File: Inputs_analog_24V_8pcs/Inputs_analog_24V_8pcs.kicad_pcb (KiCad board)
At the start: 2 copper layers, 104 parts, among them J1 Screw_Terminal_01x02, J10 Screw_Terminal_01x03, J11 Screw_Terminal_01x03, J2 Screw_Terminal_01x02, J3 Screw_Terminal_01x06, J4 Screw_Terminal_01x03, J5 Screw_Terminal_01x03, J6 Screw_Terminal_01x03, J7 Screw_Terminal_01x03, J8 Screw_Terminal_01x03, J9 Screw_Terminal_01x03, U1 SN74HC14N, U10 4N28, U11 4N28, U2 SN74HC14N, U3 74HC151N.652, U4 4N28, U5 4N28, U6 4N28, U7 4N28, U8 4N28, U9 4N28

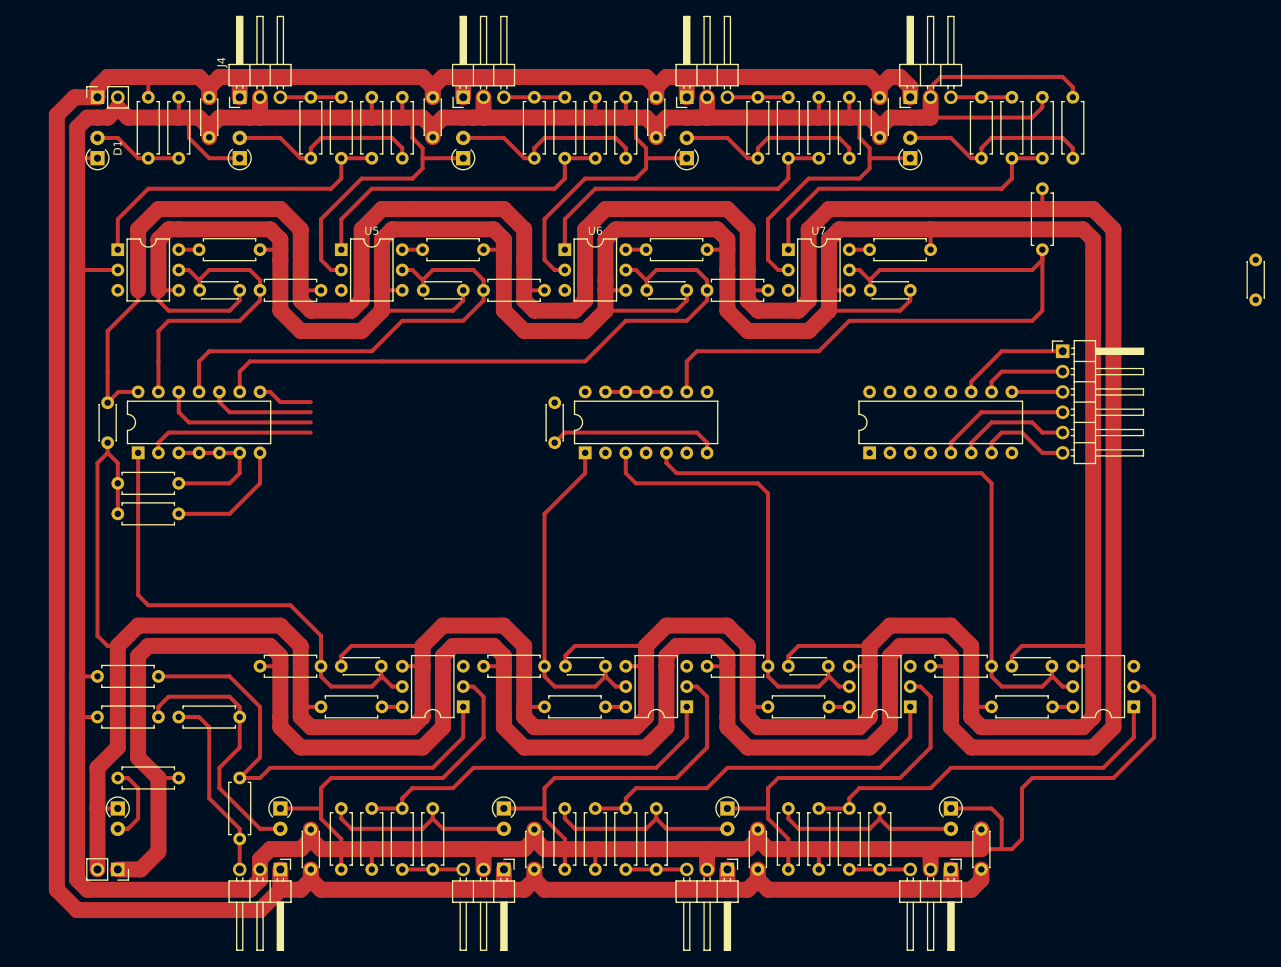
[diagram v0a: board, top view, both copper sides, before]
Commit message: Finish pcb
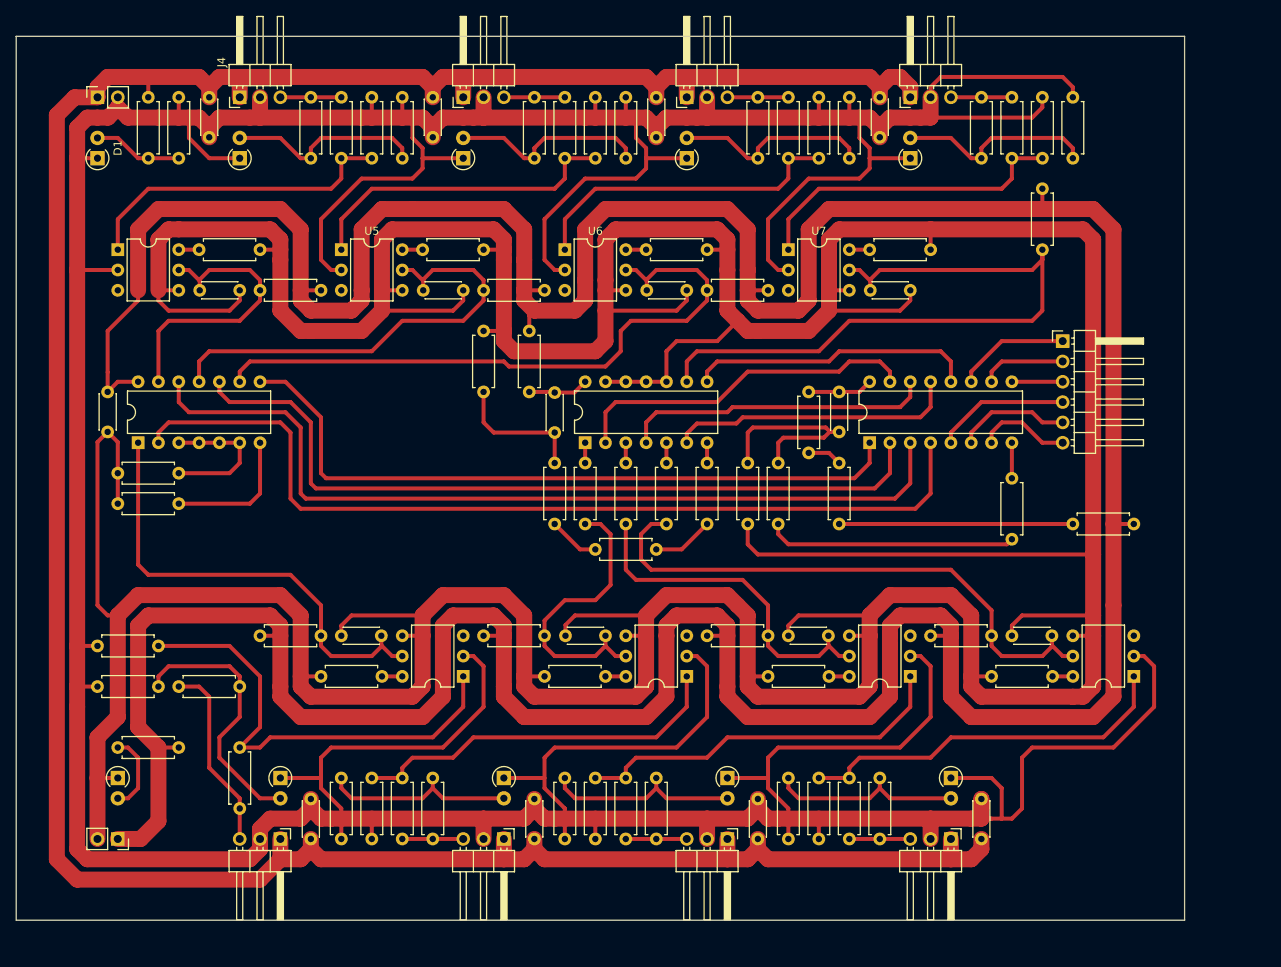
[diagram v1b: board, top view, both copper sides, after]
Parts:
- added R54: 0, Resistor_THT:R_Axial_DIN0207_L6.3mm_D2.5mm_P7.62mm_Horizontal, F.Cu at (109.2, 86.4)
- added R55: 0, Resistor_THT:R_Axial_DIN0207_L6.3mm_D2.5mm_P7.62mm_Horizontal, F.Cu at (104.1, 86.4)
- added R56: 0, Resistor_THT:R_Axial_DIN0207_L6.3mm_D2.5mm_P7.62mm_Horizontal, F.Cu at (99.1, 86.4)
- added R57: 0, Resistor_THT:R_Axial_DIN0207_L6.3mm_D2.5mm_P7.62mm_Horizontal, F.Cu at (127.0, 85.1)
- added R58: 0, Resistor_THT:R_Axial_DIN0207_L6.3mm_D2.5mm_P7.62mm_Horizontal, F.Cu at (130.8, 94.0)
- added R59: 0, Resistor_THT:R_Axial_DIN0207_L6.3mm_D2.5mm_P7.62mm_Horizontal, F.Cu at (167.6, 94.0)
- added R60: 0, Resistor_THT:R_Axial_DIN0207_L6.3mm_D2.5mm_P7.62mm_Horizontal, F.Cu at (123.2, 94.0)
- added R61: 0, Resistor_THT:R_Axial_DIN0207_L6.3mm_D2.5mm_P7.62mm_Horizontal, F.Cu at (119.4, 94.0)
- added R62: 0, Resistor_THT:R_Axial_DIN0207_L6.3mm_D2.5mm_P7.62mm_Horizontal, F.Cu at (152.4, 88.3)
- added R63: 0, Resistor_THT:R_Axial_DIN0207_L6.3mm_D2.5mm_P7.62mm_Horizontal, F.Cu at (92.1, 69.8)
- added R64: 0, Resistor_THT:R_Axial_DIN0207_L6.3mm_D2.5mm_P7.62mm_Horizontal, F.Cu at (86.4, 69.8)
- added R65: 0, Resistor_THT:R_Axial_DIN0207_L6.3mm_D2.5mm_P7.62mm_Horizontal, F.Cu at (114.3, 94.0)
- added R66: 0, Resistor_THT:R_Axial_DIN0207_L6.3mm_D2.5mm_P7.62mm_Horizontal, F.Cu at (95.2, 86.4)
- added R67: 0, Resistor_THT:R_Axial_DIN0207_L6.3mm_D2.5mm_P7.62mm_Horizontal, F.Cu at (100.3, 97.2)
- moved C3 54.6 mm to (130.8, 82.5)
- moved C11 3.81 mm to (148.6, 133.3)
- moved C12 3.81 mm to (120.7, 133.3)
- moved C14 3.81 mm to (157.4, 108.0)
- moved C15 3.81 mm to (129.5, 108.0)
- moved C16 3.81 mm to (92.7, 133.3)
- moved C17 3.81 mm to (64.8, 133.3)
- moved C18 3.81 mm to (73.6, 108.0)
- moved C19 3.81 mm to (101.6, 108.0)
- moved J10 3.81 mm to (61.0, 133.3)
- moved J11 3.81 mm to (88.9, 133.3)
- moved J2 3.81 mm to (40.6, 133.3)
- moved J8 3.81 mm to (144.8, 133.3)
- moved J9 3.81 mm to (116.8, 133.3)
- moved R27 3.81 mm to (124.5, 133.3)
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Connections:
- C2 pad 1: GND -> Net-(C2-Pad1)
- C2 pad 2: +5V -> Net-(C2-Pad2)
- C3 pad 1: GND -> Net-(C3-Pad1)
- C3 pad 2: +5V -> Net-(C3-Pad2)
- U2 pad 1: input_8 -> Net-(R56-Pad1)
- U2 pad 14: +5V -> Net-(C2-Pad2)
- U2 pad 3: input_6 -> Net-(R55-Pad1)
- U2 pad 5: input_5 -> Net-(R54-Pad1)
- U2 pad 7: GND -> Net-(R65-Pad2)
- U3 pad 12: Net-(U3-Pad12) -> Net-(U2-Pad8)
- U3 pad 13: Net-(U3-Pad13) -> Net-(U2-Pad6)
- U3 pad 14: Net-(U1-Pad12) -> Net-(U2-Pad4)
- U3 pad 15: Net-(U1-Pad10) -> Net-(U2-Pad2)
- U3 pad 16: +5V -> Net-(C3-Pad2)
- U3 pad 2: Net-(U3-Pad2) -> Net-(U1-Pad10)
- U3 pad 3: Net-(U3-Pad3) -> Net-(U1-Pad12)
- U3 pad 8: GND -> Net-(R62-Pad1)
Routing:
- net Net-(U1-Pad2): track 20.8 -> 114.8 mm
- net Net-(U1-Pad12): track 19.6 -> 109.7 mm
- net Net-(U1-Pad10): track 13.2 -> 99.2 mm
- net Net-(U1-Pad8): track 6.88 -> 88.6 mm
- net Net-(U2-Pad2): track 0.00 -> 43.8 mm
- net GND: track 678.0 -> 721.3 mm
- net Net-(U2-Pad4): track 0.00 -> 38.8 mm
- net Net-(U2-Pad6): track 0.00 -> 36.2 mm
- net Net-(U2-Pad8): track 0.00 -> 35.9 mm
- net Net-(R60-Pad1): track 0.00 -> 31.3 mm
- net Net-(R58-Pad1): track 0.00 -> 29.2 mm
- net Net-(C3-Pad1): track 0.00 -> 25.3 mm
- net Net-(C2-Pad1): track 0.00 -> 17.0 mm
- net input_6: track 57.3 -> 43.5 mm
- net input_5: track 80.2 -> 70.9 mm
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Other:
- board outline added: 146.1 x 110.5 mm
